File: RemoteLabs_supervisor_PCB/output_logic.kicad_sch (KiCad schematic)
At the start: 44 parts

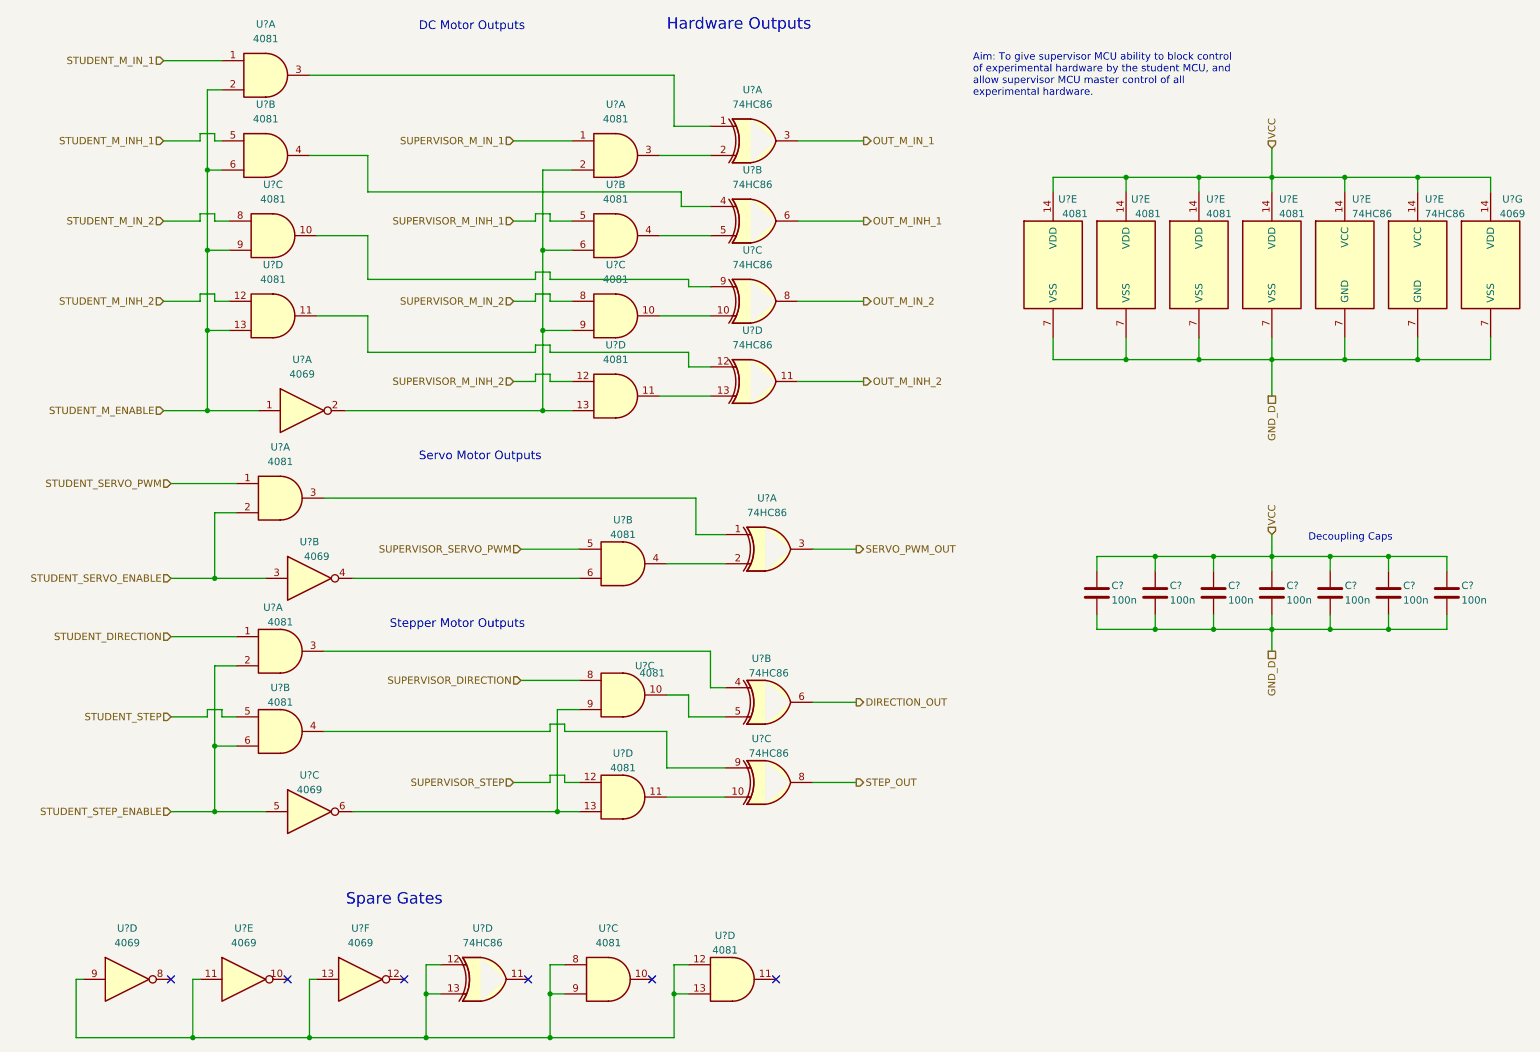
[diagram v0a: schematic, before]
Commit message: lunchtime backup
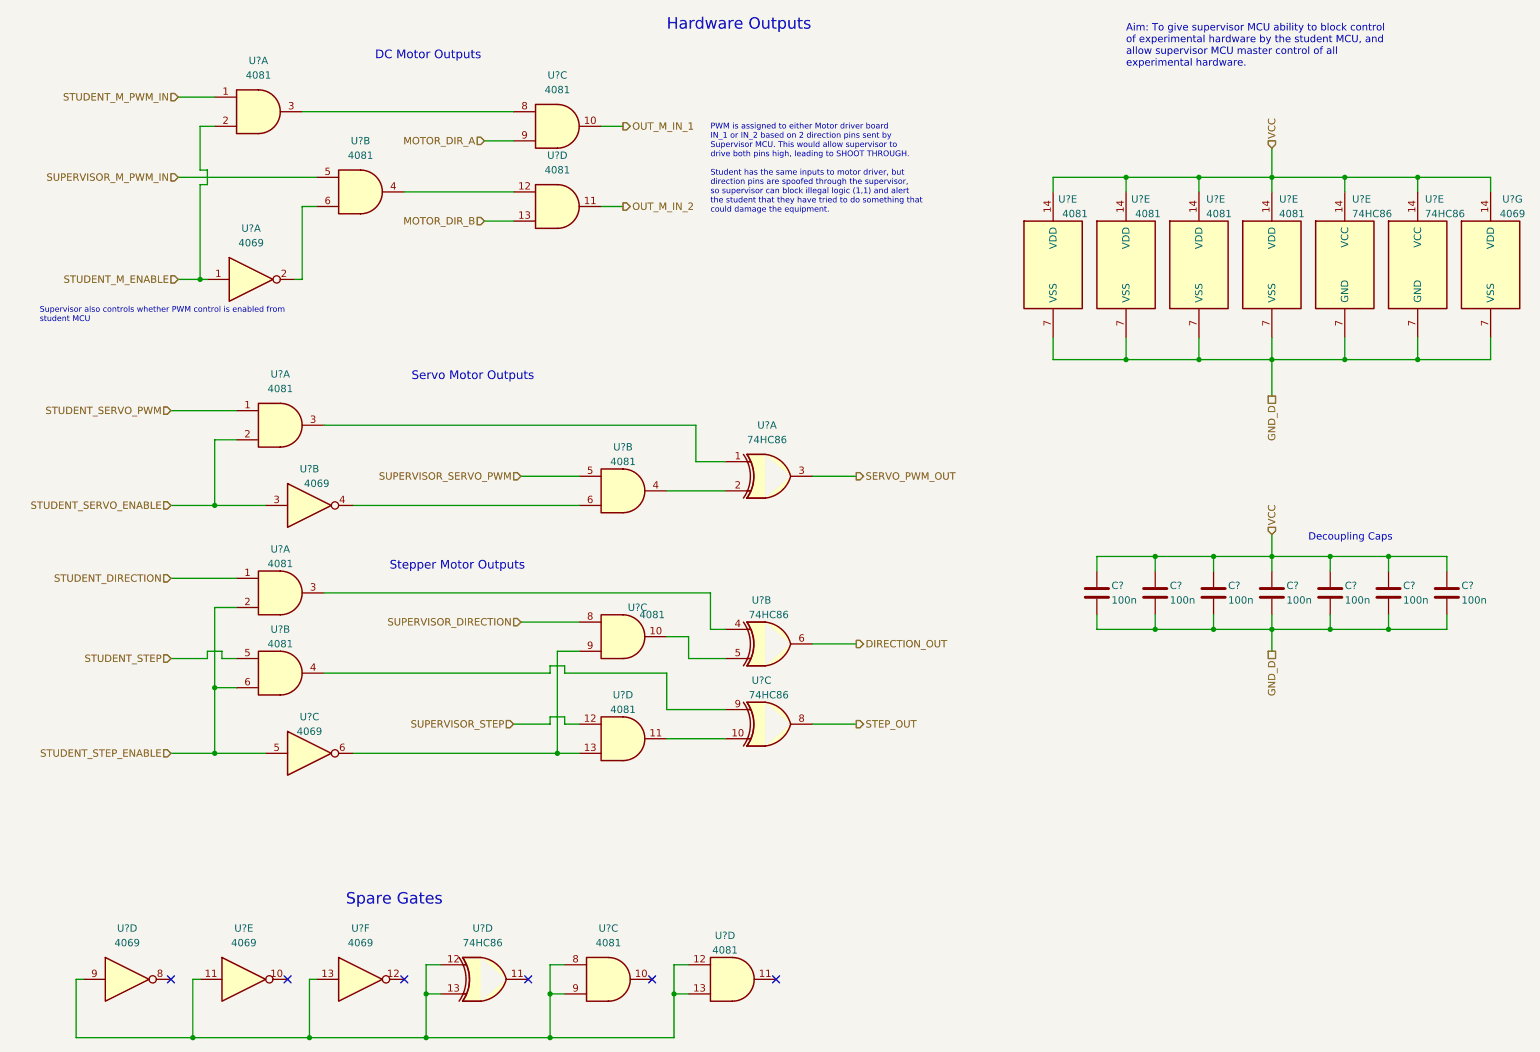
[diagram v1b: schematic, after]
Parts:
- removed U? (x4): 74HC86, symbol 74xx:74HC86
- removed U? (x4): 4081, symbol 4xxx:4081
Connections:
- net STUDENT_M_INH_2 is gone; now on an unnamed net: U?.12
- net STUDENT_M_IN_2 is gone; now on an unnamed net: U?.8
- net OUT_M_IN_1: now also U?.10
- net OUT_M_IN_2: now also U?.11
- net STUDENT_M_ENABLE: no longer U?.13, U?.6, U?.9
- net at U?.2: now also U?.6
- net STUDENT_M_INH_1 renamed SUPERVISOR_M_PWM_IN
- net STUDENT_M_IN_1 renamed STUDENT_M_PWM_IN
- new net MOTOR_DIR_A: U?.9
- new net MOTOR_DIR_B: U?.13
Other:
- note added: "PWM is assigned to either Motor driver board IN_1 or IN_2 based on 2 direction pins sent by Supervisor MCU. This would allow supervisor to drive both pins high, leading to SHOOT THROUGH. Student has the same inputs to motor driver, but direction pins are spoofed through the supervisor, so supervisor can block illegal logic (1,1) and alert the student that they have tried to do something that coul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"
- note added: "Supervisor also controls whether PWM control is enabled from student MCU"
- moved on the sheet: U?A, U?B, U?C, U?D
